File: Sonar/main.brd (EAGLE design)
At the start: 10 parts, among them IC1 4066N, Q1 BC488

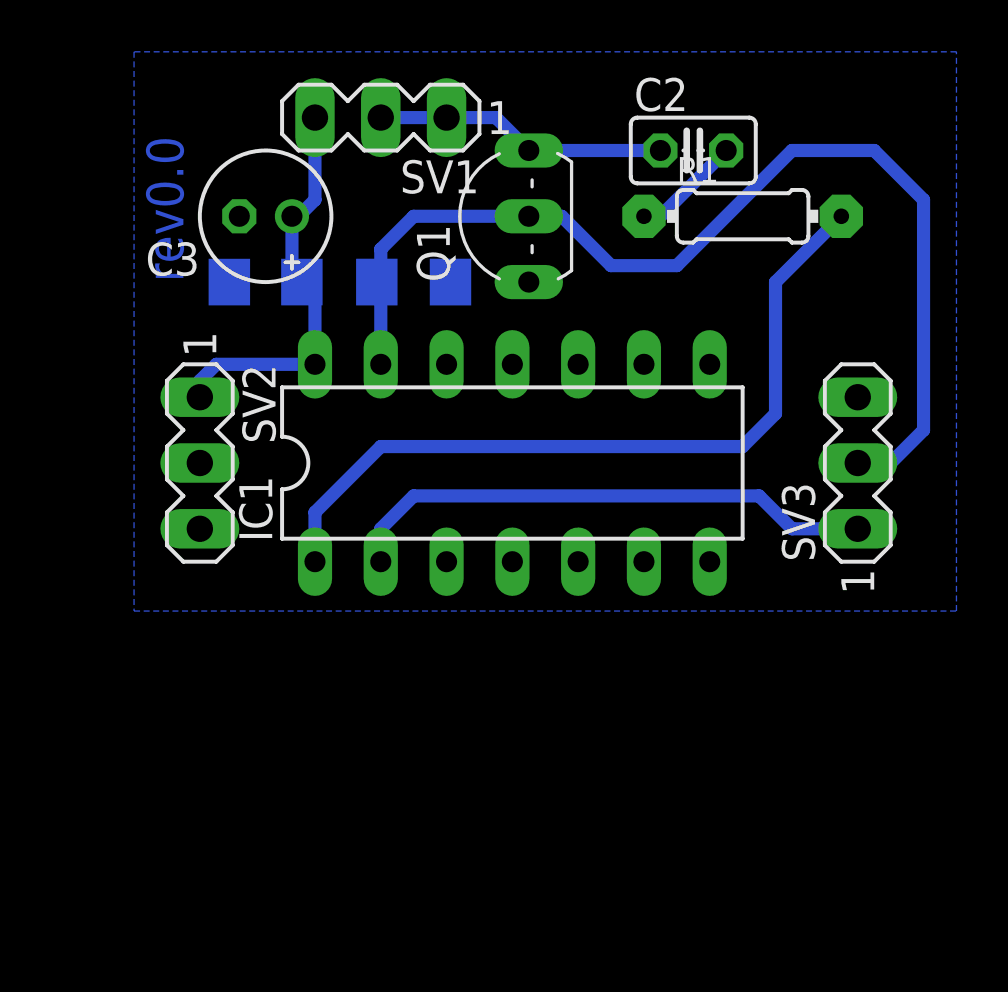
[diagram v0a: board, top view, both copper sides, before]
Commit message: Minor layout changes.
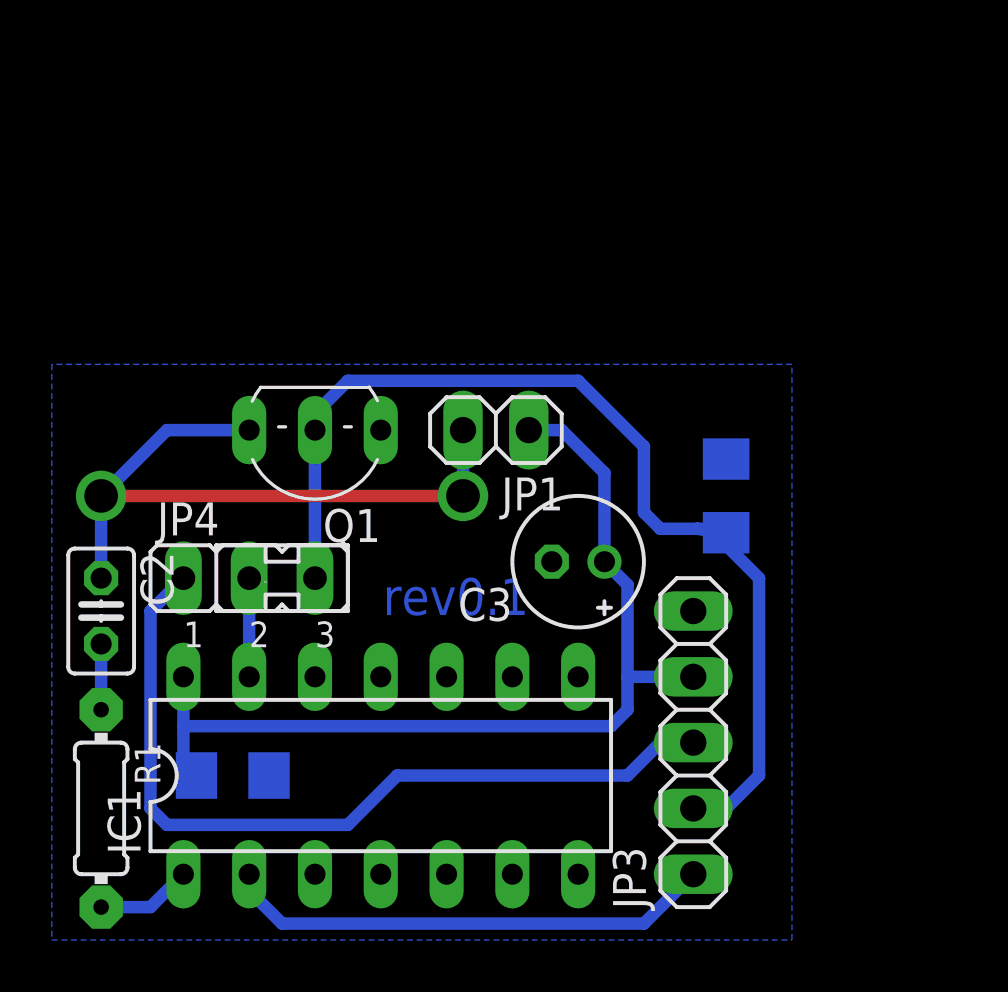
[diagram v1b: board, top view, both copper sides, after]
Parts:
- removed SV1, SV2, SV3: (no value), con-lstb:MA03-1
- added J1: (no value), jumper:JUMP
- added JP1: (no value), pinhead:1X02
- added JP3: (no value), pinhead:1X05
- added JP4: (no value), jumper:JP2
- C1: value (none) -> 100n
- C2: value (none) -> 220n
- C3: value (none) -> 100u
- R1: value (none) -> 470R
- R2: value (none) -> 2k2
- moved R1 33.7 mm to (1.91, 5.08), turned to 270 degrees
- moved C2 29.0 mm to (1.91, 12.7), turned to 270 degrees
- moved C1 19.1 mm to (6.99, 6.35), turned to 180 degrees
- moved C3 18.0 mm to (20.3, 14.6)
- moved R2 14.6 mm to (26.0, 17.1), turned to 270 degrees
- moved IC1 13.1 mm to (12.7, 6.35)
- moved Q1 11.8 mm to (10.2, 18.4), turned to 180 degrees
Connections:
- removed net N$1: IC1.13, Q1.B, R2.2, SV3.2
- removed net N$2: IC1.2, SV3.1
- new net N$8: IC1.13, JP4.2
- new net OUT: IC1.2, JP3.1
- new net OUT-ENABLE: JP3.3, JP4.1
- new net SPEAKER-IN: JP3.2, JP4.3, Q1.B, R2.2
- net GND: now also JP3.5; no longer SV2.2, SV2.3, SV3.3
- net N$3: now also JP1.2; no longer SV1.1, SV1.2
- net VCC: now also JP1.1, JP3.4; no longer SV1.3, SV2.1
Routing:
- net N$1: track 41.5 -> 0.00 mm
- net SPEAKER-IN: track 0.00 -> 40.5 mm
- net OUT-ENABLE: track 0.00 -> 31.9 mm
- net N$5: track 29.9 -> 3.70 mm
- net VCC: track 15.8 -> 37.1 mm
- net N$2: track 20.7 -> 0.00 mm
- net OUT: track 0.00 -> 19.1 mm
- net N$3: track 11.3 -> 26.5 mm, vias 0 -> 2
- net N$8: track 0.00 -> 3.81 mm
- net N$4: track 4.23 -> 2.54 mm
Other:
- board text added: "rev0.1"
- board text removed: "rev0.0"
